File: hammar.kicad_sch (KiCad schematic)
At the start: 116 parts, among them J1 8x screw terminal, 5,08mm spa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, J10 1x2, J11 1x4, J12 1x3, J13 1x8, J14 1x3, J15 1x3, J16 1x3, J2 Micro_SD_Holder, J3 USB_C_Receptacle_USB2.0, J4 1x4, J5 1x4, J6 1x4, J7 1x4, J8 1x4, J9 1x2, Q1 S9014 or equivalent, Q2 S9014 or equivalent, Q3 TI CSD17310Q5A or equivalent, Q4 PMV40UN2R or equivalent, Q5 PMV40UN2R or equivalent, SW1 SW_MEC_5G, U1 A4988, U2 A4988, U3 A4988, U4 A4988, U5 DPAK 3,3v linear regulator + 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, U6 ESP32-WROOM-32E, U7 CH340G, Y1 Resonator_12mhz

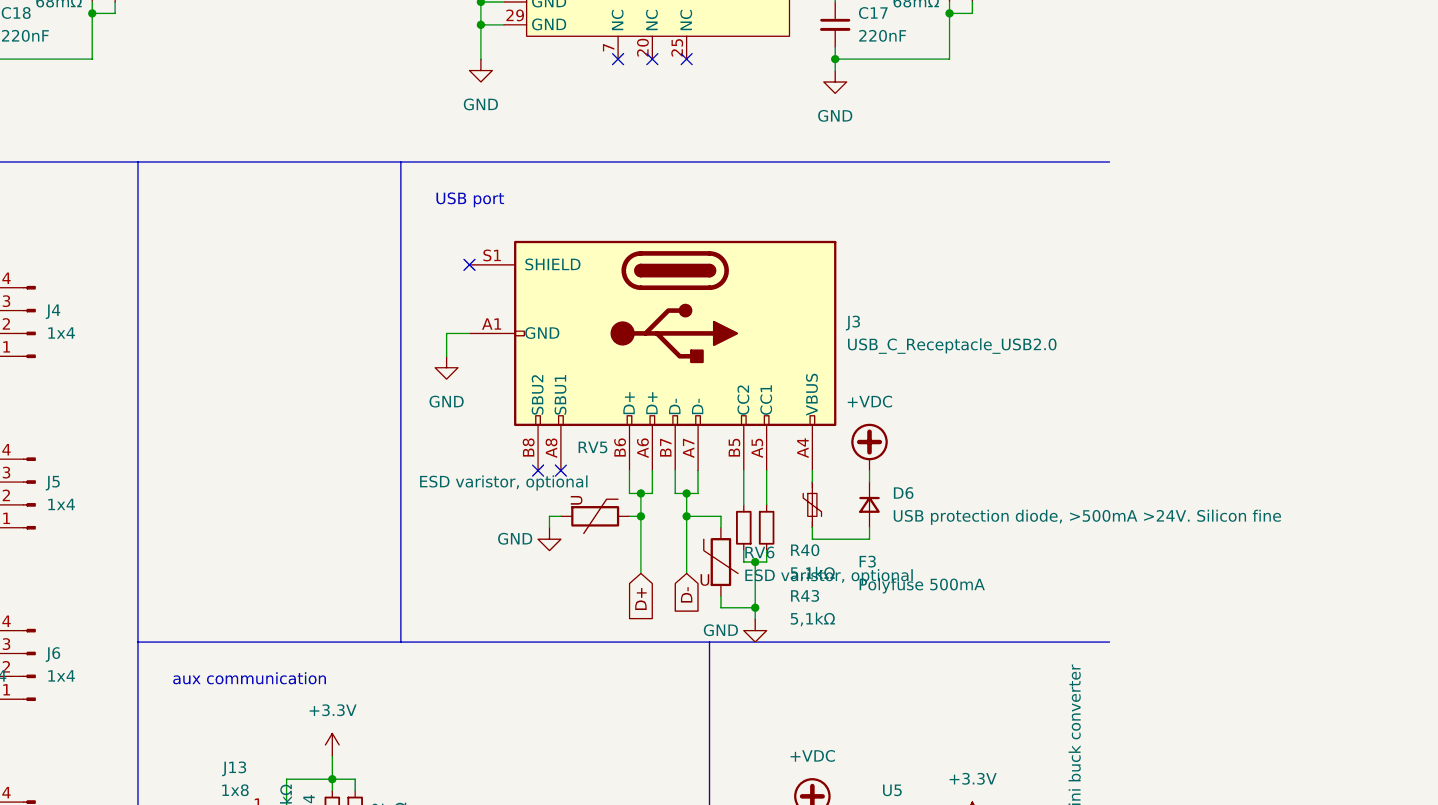
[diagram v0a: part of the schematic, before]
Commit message: slight reference update
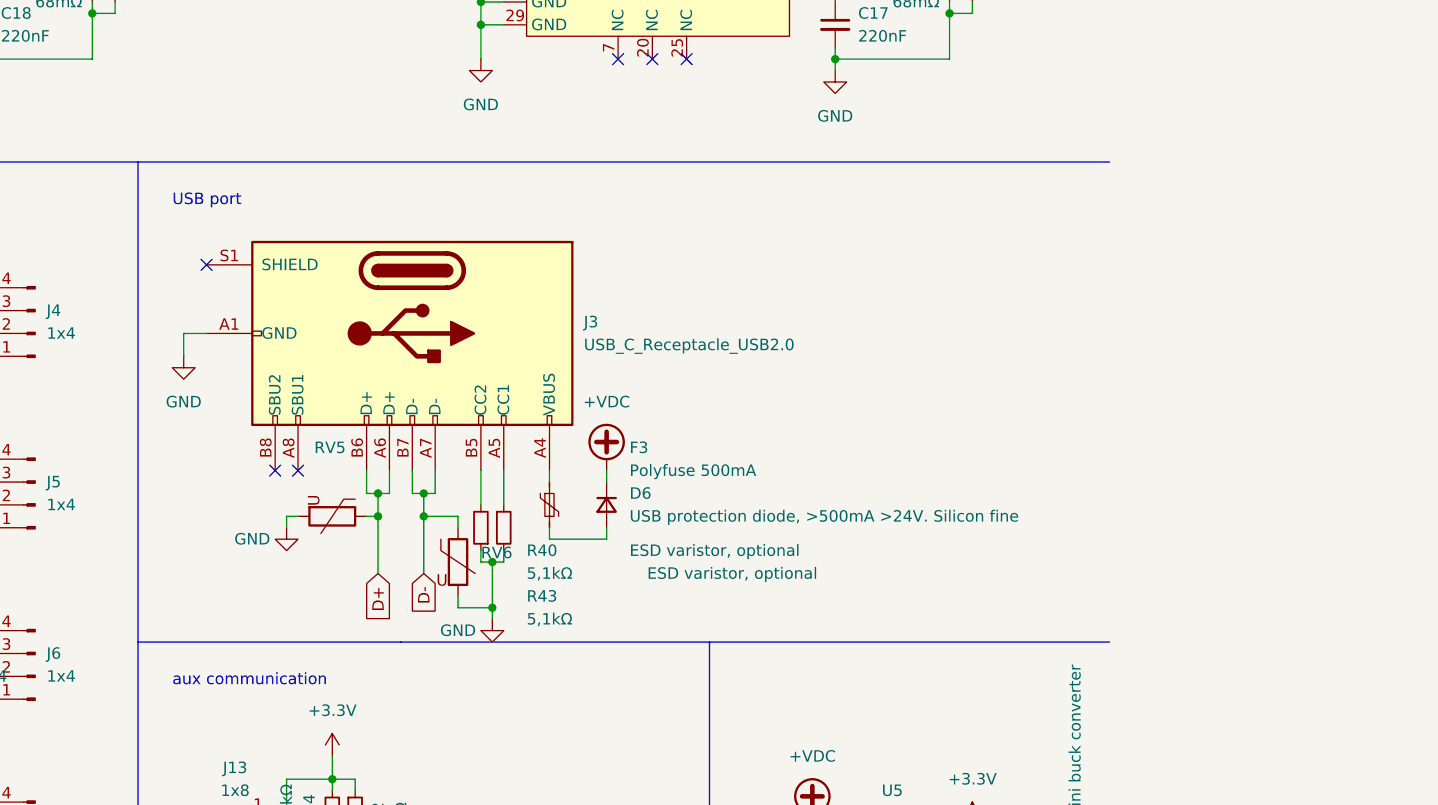
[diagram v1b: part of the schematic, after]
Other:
- moved on the sheet: D6, F3, J3, R40, R43, RV5, RV6

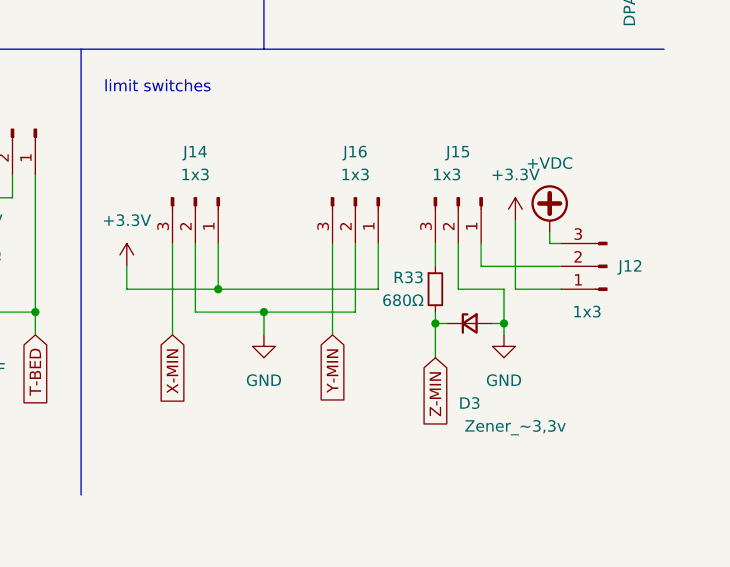
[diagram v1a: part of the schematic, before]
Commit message: BOM++
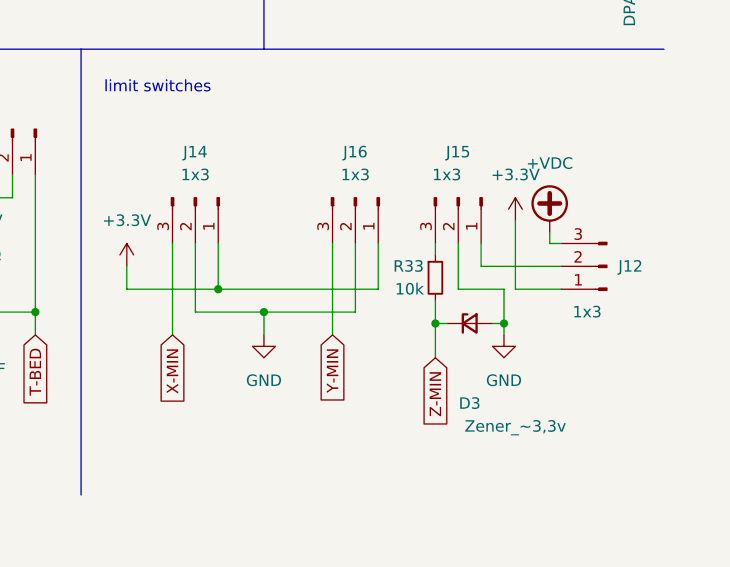
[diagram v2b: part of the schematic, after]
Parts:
- R33: value 680Ω -> 10k
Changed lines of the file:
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@@
     (stroke (width 0) (type default) (color 0 0 0 0))
   )
-  (wire (pts (xy 382.27 224.79) (xy 382.27 227.33))
+  (wire (pts (xy 382.27 224.79) (xy 382.27 226.06))
     (stroke (width 0) (type default) (color 0 0 0 0))
   )
@@
     (stroke (width 0) (type default) (color 0 0 0 0))
   )
+  (wire (pts (xy 382.27 231.14) (xy 382.27 233.68))
+    (stroke (width 0) (type default) (color 0 0 0 0))
+  )
   (wire (pts (xy 97.79 274.32) (xy 97.79 275.59))
     (stroke (width 0) (type default) (color 0 0 0 0))
@@
     (stroke (width 0) (type default) (color 0 0 0 0))
   )
-  (wire (pts (xy 382.27 233.68) (xy 382.27 232.41))
-    (stroke (width 0) (type default) (color 0 0 0 0))
-  )
   (wire (pts (xy 353.06 224.79) (xy 353.06 234.95))
     (stroke (width 0) (type default) (color 0 0 0 0))
@@
     (pin "2")
   )
-  (symbol (lib_id "Device:R_Small") (at 382.27 229.87 0) (unit 1)
-    (in_bom yes) (on_board yes)
-    (property "Reference" "R33" (id 0) (at 381 228.6 0)
-      (effects (font (size 1.27 1.27)) (justify right))
-    )
-    (property "Value" "680Ω" (id 1) (at 381 231.14 0)
-      (effects (font (size 1.27 1.27)) (justify right))
-    )
-    (property "Footprint" "Resistor_SMD:R_0603_1608Metric" (id 2) (at 382.27 229.87 0)
-      (effects (font (size 1.27 1.27)) hide)
-    )
-    (property "Datasheet" "~" (id 3) (at 382.27 229.87 0)
-      (effects (font (size 1.27 1.27)) hide)
-    )
-    (pin "1")
-    (pin "2")
-  )
   (symbol (lib_id "Device:R_Small") (at 229.87 27.94 0) (unit 1)
     (in_bom yes) (on_board yes)
@@
     (pin "1")
   )
+  (symbol (lib_id "Device:R_Small") (at 382.27 228.6 0) (unit 1)
+    (in_bom yes) (on_board yes)
+    (property "Reference" "R33" (id 0) (at 381 227.33 0)
+      (effects (font (size 1.27 1.27)) (justify right))
+    )
+    (property "Value" "10k" (id 1) (at 381 229.87 0)
+      (effects (font (size 1.27 1.27)) (justify right))
+    )
+    (property "Footprint" "Resistor_SMD:R_0603_1608Metric" (id 2) (at 382.27 228.6 0)
+      (effects (font (size 1.27 1.27)) hide)
+    )
+    (property "Datasheet" "~" (id 3) (at 382.27 228.6 0)
+      (effects (font (size 1.27 1.27)) hide)
+    )
+    (pin "1")
+    (pin "2")
+  )
   (symbol (lib_id "Device:R_Small") (at 273.05 261.62 180) (unit 1)
     (in_bom yes) (on_board yes)
@@
       (reference "R32") (unit 1) (value "10kΩ") (footprint "Resistor_SMD:R_0603_1608Metric")
     )
-    (path "/31f81989-9b57-4f02-b45c-ef1741cf0df2"
-      (reference "R33") (unit 1) (value "680Ω") (footprint "Resistor_SMD:R_0603_1608Metric")
+    (path "/b56c360d-4c22-478e-8f02-968635d4cfa3"
+      (reference "R33") (unit 1) (value "10k") (footprint "Resistor_SMD:R_0603_1608Metric")
     )
     (path "/536fa290-c4ad-4563-8eae-3e2b761794e3"
